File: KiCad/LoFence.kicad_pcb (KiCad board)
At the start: 2 copper layers, 72 x 133 mm, 73 parts, among them J1 Fence+, J2 Fence-, J3 ISP, J5 DEBUG MCU, J6 DEBUG LA, J7 FLASH LA, Q1 LBSS84LT1G, Q2 2N7002, U1 TPS63051RMW, U2 TLV9062, U3 ATmega328PB-AU, U4 LA66, Y1 32768 Hz

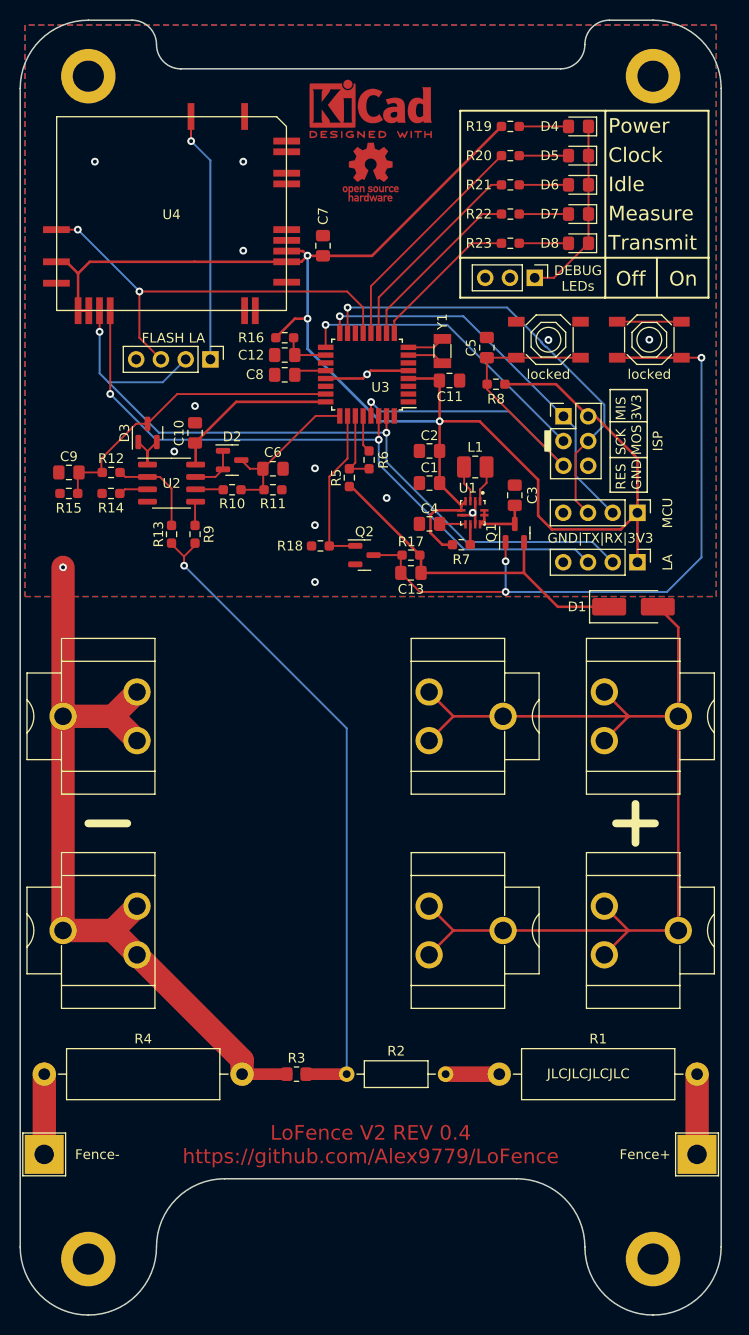
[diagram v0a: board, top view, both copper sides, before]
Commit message: move battery clamps to avoid overlapping with case screw holes
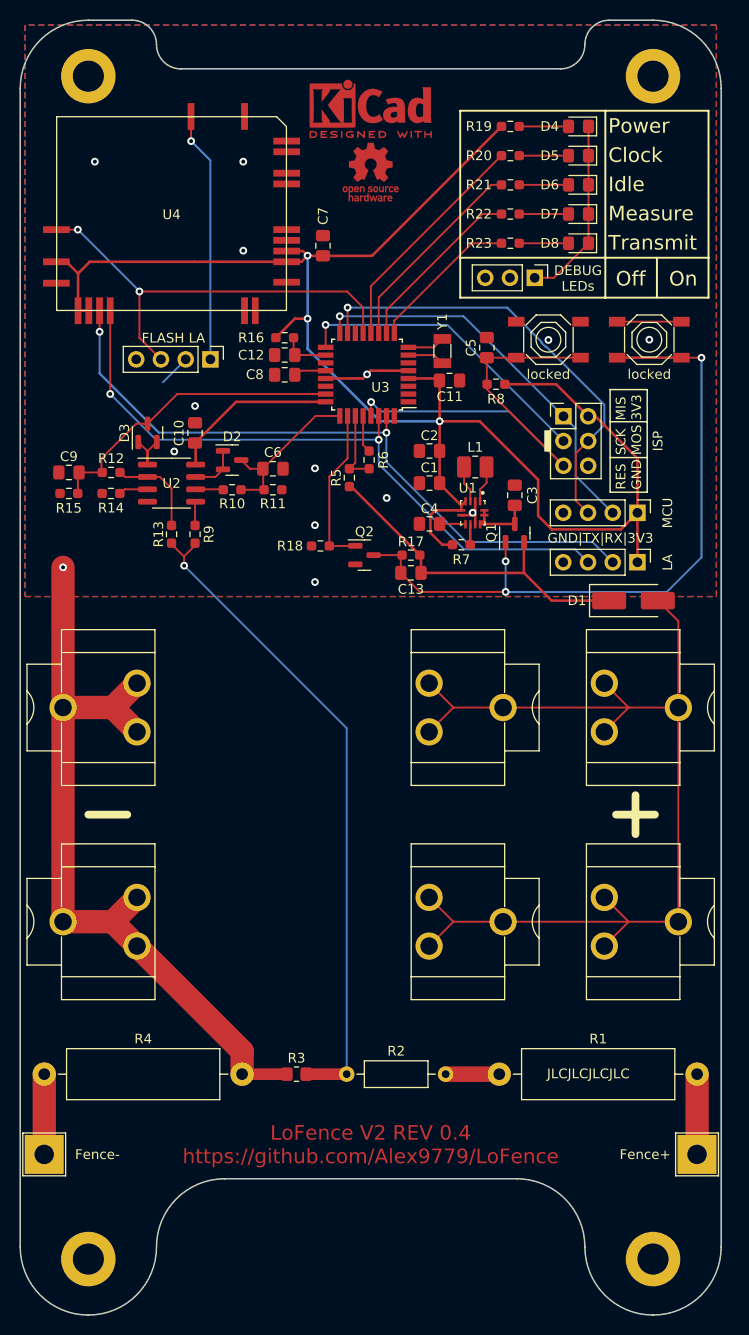
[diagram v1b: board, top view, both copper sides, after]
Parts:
- moved B10 0.90 mm to (47.0, 105.6)
- moved B11 0.90 mm to (95.0, 105.6)
- moved B20 0.90 mm to (47.0, 127.6)
- moved B21 0.90 mm to (95.0, 127.6)
- moved B31 0.90 mm to (77.0, 105.6)
- moved B41 0.90 mm to (77.0, 127.6)
- moved D1 0.64 mm to (98.0, 94.6)
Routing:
- net LA_RX: track 79.6 -> 82.6 mm
